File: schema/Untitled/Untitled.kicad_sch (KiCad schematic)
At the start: 10 parts, among them SW1 SW_Push, SW2 SW_Push, U1 ATtiny84A-P, U2 74HC595, U3 74HC595, U4 CC56-12SURKWA

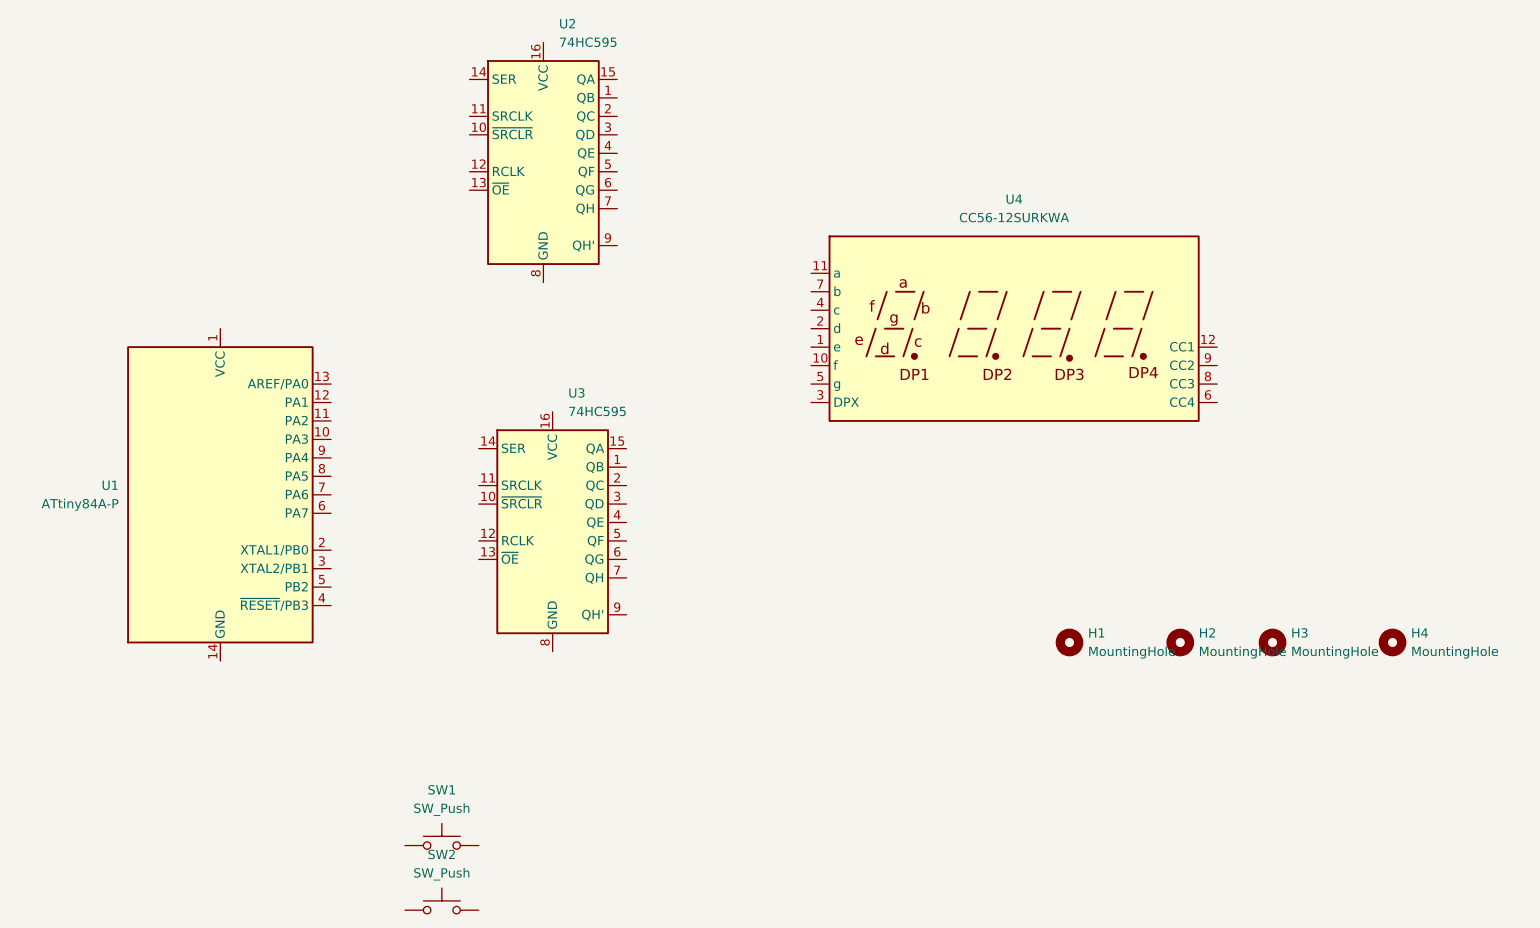
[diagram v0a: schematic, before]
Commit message: version funcional 1
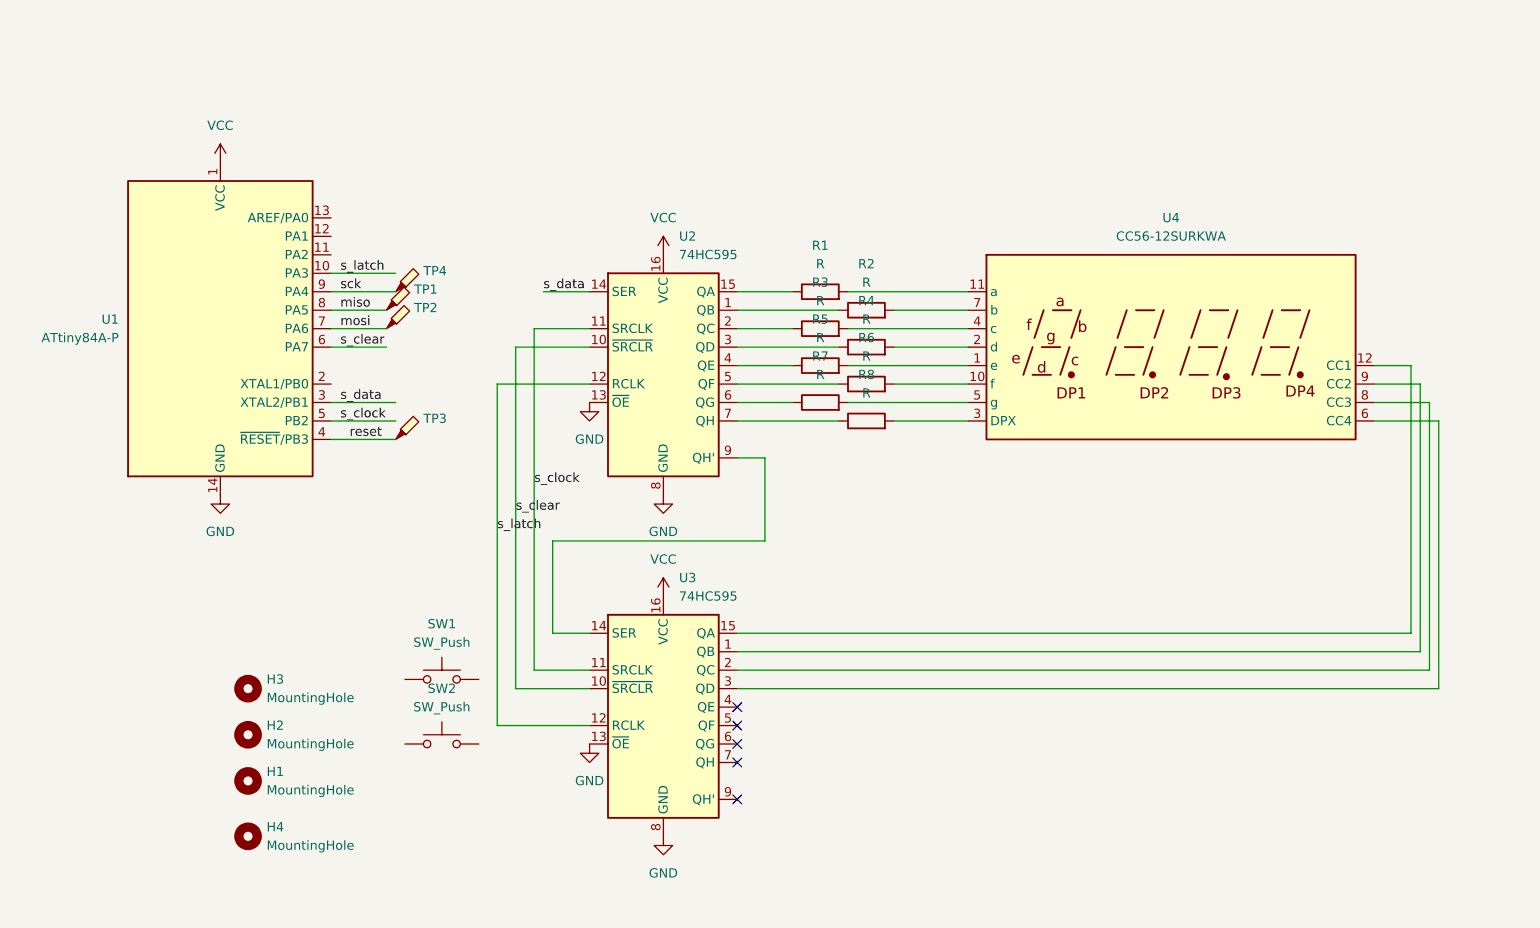
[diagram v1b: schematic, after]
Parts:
- added R1, R2, R3, R4, R5, R6, R7, R8: R, symbol Device:R
- added TP1, TP2, TP3, TP4: TestPoint_Probe, Connector_Pin:Pin_D1.0mm_L10.0mm, symbol Connector:TestPoint_Probe
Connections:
- net VCC: now reaches U1.1 (VCC)
- net VCC: now also U2.16 (VCC), U3.16 (VCC)
- net s_latch: now reaches U1.10 (PA3)
- net s_latch: now also U2.12 (RCLK), U3.12 (RCLK)
- net GND: now reaches U1.14 (GND)
- net GND: now also U2.13 (~{OE}), U2.8 (GND), U3.13 (~{OE}), U3.8 (GND)
- net s_data: now reaches U1.3 (XTAL2/PB1)
- net s_data: now also U2.14 (SER)
- net reset: now reaches U1.4 (~{RESET}/PB3)
- net reset: now also TP3.1
- net s_clock: now reaches U1.5 (PB2)
- net s_clock: now also U2.11 (SRCLK), U3.11 (SRCLK)
- net s_clear: now reaches U1.6 (PA7)
- net s_clear: now also U2.10 (~{SRCLR}), U3.10 (~{SRCLR})
- net mosi: now reaches U1.7 (PA6)
- net mosi: now also TP2.1
- net miso: now reaches U1.8 (PA5)
- net miso: now also TP1.1
- net sck: now reaches U1.9 (PA4)
- net sck: now also TP4.1
- net at U4.1 (e): now also R5.2
- net at U4.10 (f): now also R6.2
- net at U4.11 (a): now also R1.2
- net at U4.12 (CC1): now also U3.15 (QA)
- net at U4.2 (d): now also R4.2
- net at U4.3 (DPX): now also R8.2
- net at U4.4 (c): now also R3.2
- net at U4.5 (g): now also R7.2
- net at U4.6 (CC4): now also U3.3 (QD)
- net at U4.7 (b): now also R2.2
- net at U4.8 (CC3): now also U3.2 (QC)
- net at U4.9 (CC2): now also U3.1 (QB)
- net at U3.14 (SER): now also U2.9 (QH')
- net at U2.1 (QB): now also R2.1
- net at U2.15 (QA): now also R1.1
- net at U2.2 (QC): now also R3.1
- net at U2.3 (QD): now also R4.1
- net at U2.4 (QE): now also R5.1
- net at U2.5 (QF): now also R6.1
- net at U2.6 (QG): now also R7.1
- net at U2.7 (QH): now also R8.1
- no-connect marks 0 -> 5
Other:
- moved on the sheet: H1, H2, H3, H4, SW1, SW2, U1, U2, U3, U4
